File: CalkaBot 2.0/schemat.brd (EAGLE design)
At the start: 94.4 x 101.8 mm, 56 parts, among them IC1 TB6612FNG, IC2 LM339D, IC3 7806DT, Q1 16MHz

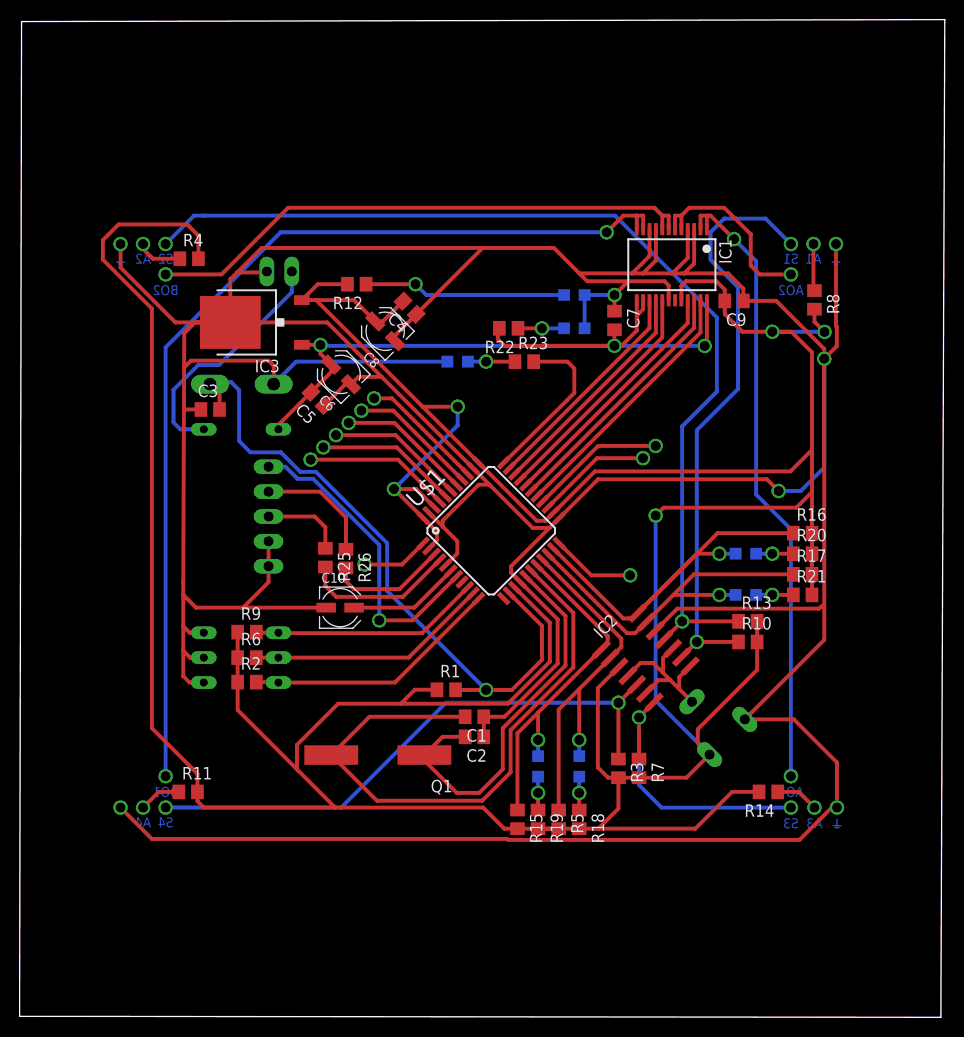
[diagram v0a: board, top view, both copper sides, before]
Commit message: chyba skończyłem
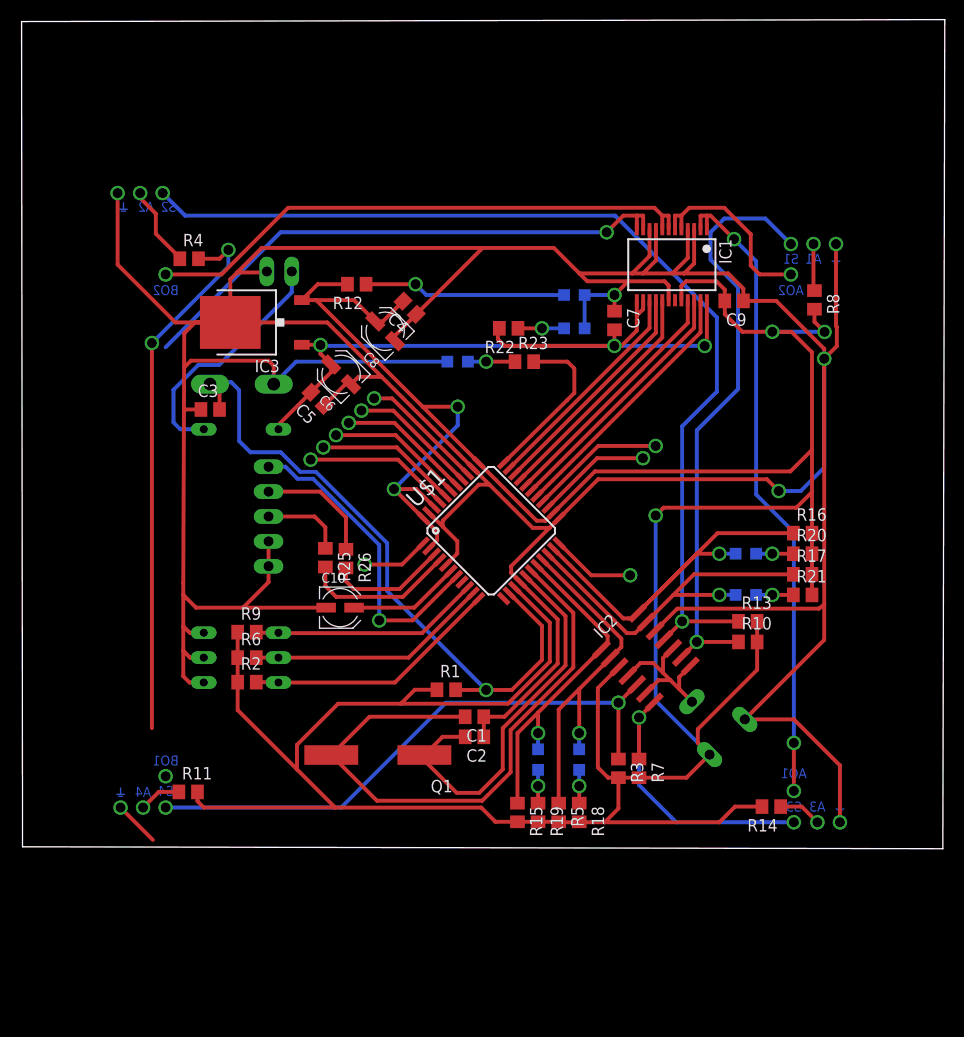
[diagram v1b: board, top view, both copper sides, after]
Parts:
- added U$3: (no value), untitled:GND@1
- moved U$5 5.41 mm to (12.7, 71.4)
- moved U$2 1.73 mm to (85.8, 10.2)
- moved R14 1.53 mm to (78.8, 10.3)
- moved LED1 0.70 mm to (59.2, 15.1)
- moved LED2 0.70 mm to (55.0, 15.1)
- moved R15 0.70 mm to (52.9, 9.70)
- moved R18 0.70 mm to (59.2, 9.70)
- moved R19 0.70 mm to (55.0, 9.70)
- moved R5 0.70 mm to (57.1, 9.70)
- moved U$4 0.10 mm to (85.4, 66.1)
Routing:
- net GND: track 545.0 -> 481.3 mm
- net BO1: track 100.8 -> 57.1 mm
- net VCC: track 454.4 -> 432.6 mm, vias 5 -> 7
- net N$1: track 4.66 -> 8.38 mm
- net AO1: track 64.4 -> 66.0 mm, vias 2 -> 3
- net FL1: track 38.5 -> 37.1 mm
- net FL2: track 36.2 -> 34.8 mm
- net S2: track 29.8 -> 30.7 mm
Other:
- board size 94.4 x 101.8 mm -> 94.2 x 84.6 mm
